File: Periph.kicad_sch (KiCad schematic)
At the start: 11 parts, among them U10 ICM-42688-P, U9 W25Q128JVS

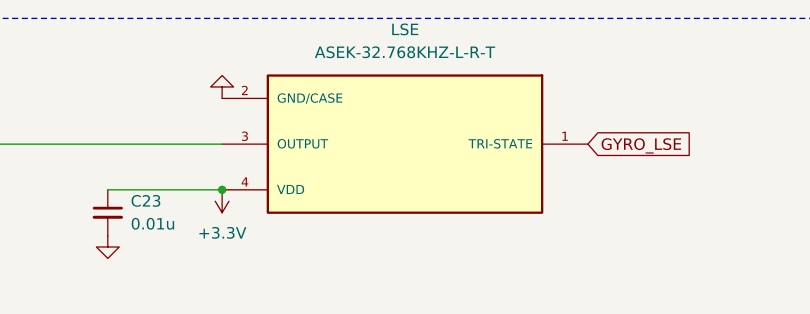
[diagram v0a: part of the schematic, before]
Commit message: update
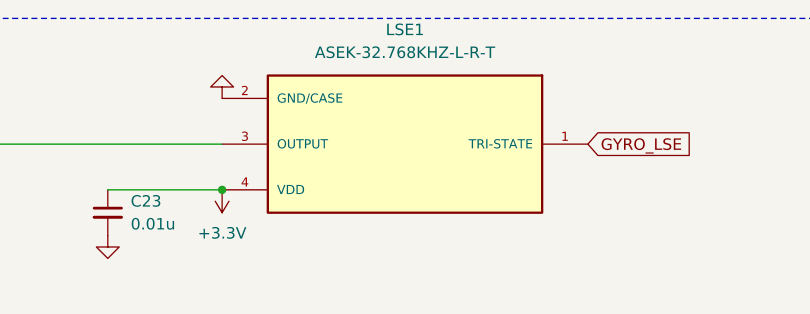
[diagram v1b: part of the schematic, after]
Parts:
- renumbered LSE to LSE1
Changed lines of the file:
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@@
 		(dnp no)
 		(fields_autoplaced yes)
-		(property "Reference" "LSE"
+		(property "Reference" "LSE1"
 			(at 109.22 20.32 0)
 			(effects
@@
 			(project ""
 				(path "/8ed38441-7d4e-4e89-870f-07e11c6dce38/57f4b5bf-da86-4b65-9b05-7c9ef99c472c"
-					(reference "LSE")
+					(reference "LSE1")
 					(unit 1)
 				)
